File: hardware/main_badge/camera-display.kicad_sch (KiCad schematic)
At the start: 6 parts, among them J3 ILI9341 Display Module, J4 OV2640 Camera Module, Q1 2N7002

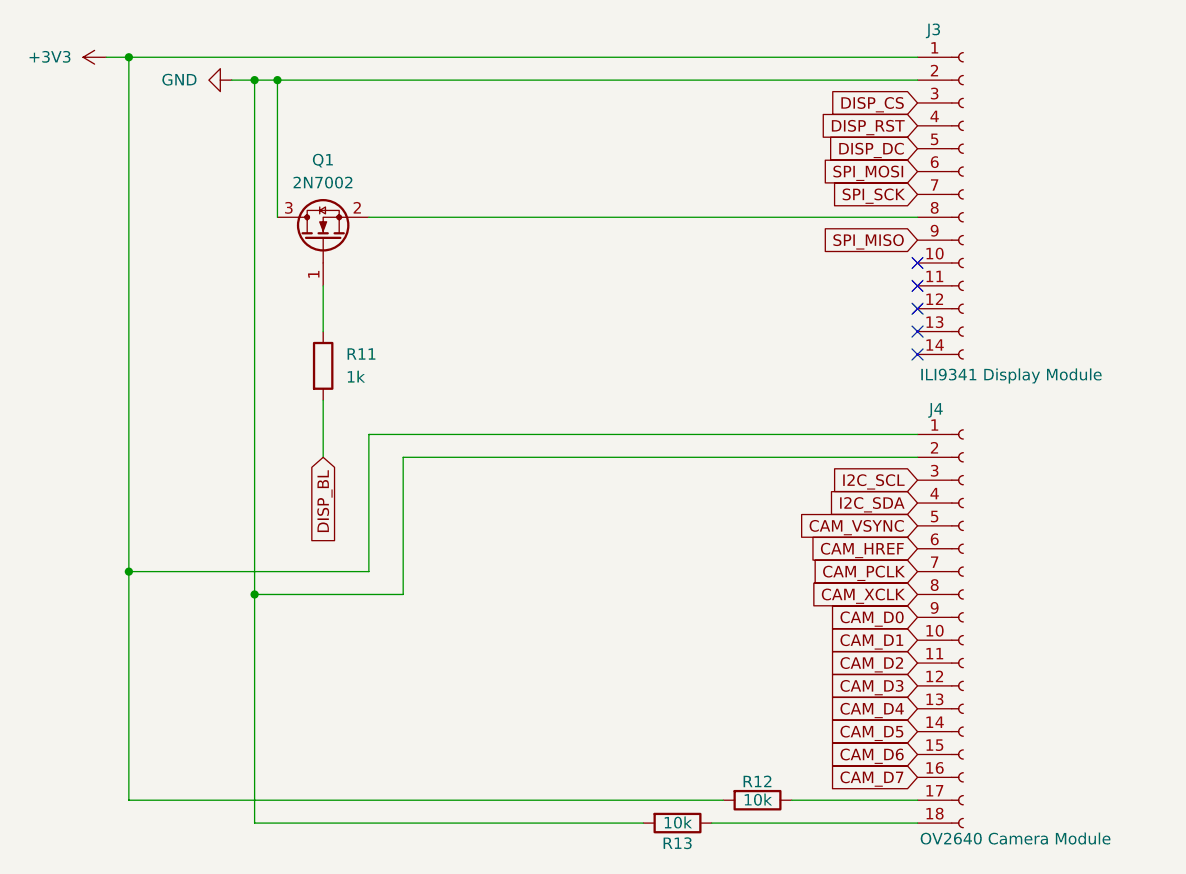
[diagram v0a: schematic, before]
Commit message: main board done except for placing LEDs and drawing ears... I think
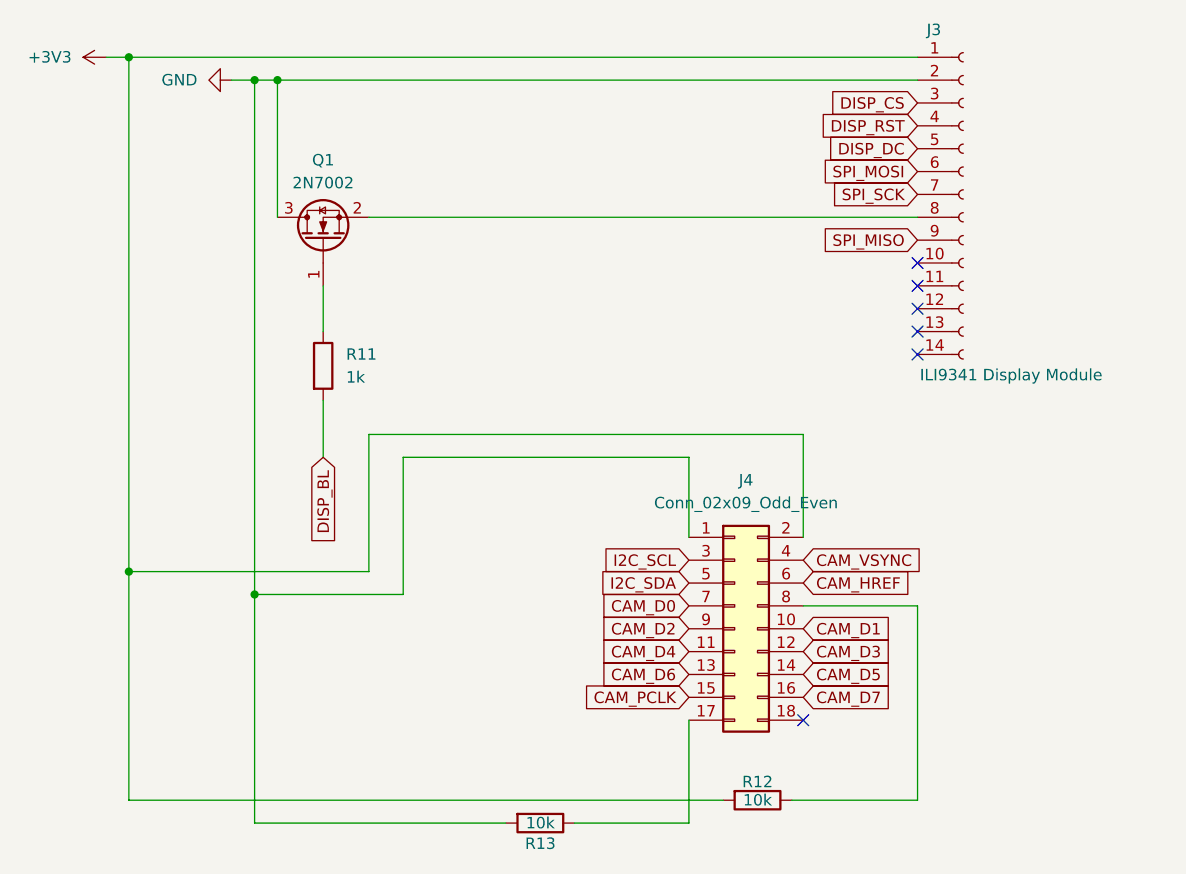
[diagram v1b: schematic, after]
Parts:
- removed J4: OV2640 Camera Module, Connector_PinSocket_2.54mm:PinSocket_1x18_P2.54mm_Vertical, symbol Connector:Conn_01x18_Socket
- added J4: Conn_02x09_Odd_Even, Connector_PinSocket_2.54mm:PinSocket_2x09_P2.54mm_Vertical, symbol Connector_Generic:Conn_02x09_Odd_Even
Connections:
- net +3V3: now also J4.2 (Pin_2)
- net CAM_D0: now also J4.7 (Pin_7)
- net CAM_D1: now also J4.10 (Pin_10)
- net CAM_D2: now also J4.9 (Pin_9)
- net CAM_D3: now also J4.12 (Pin_12)
- net CAM_D4: now also J4.11 (Pin_11)
- net CAM_D5: now also J4.14 (Pin_14)
- net CAM_D6: now also J4.13 (Pin_13)
- net CAM_D7: now also J4.16 (Pin_16)
- net CAM_HREF: now also J4.6 (Pin_6)
- net CAM_PCLK: now also J4.15 (Pin_15)
- net CAM_VSYNC: now also J4.4 (Pin_4)
- net GND: now also J4.1 (Pin_1)
- net I2C_SCL: now also J4.3 (Pin_3)
- net I2C_SDA: now also J4.5 (Pin_5)
- net at R12.1: now also J4.8 (Pin_8)
- net at R13.1: now also J4.17 (Pin_17)
- no-connect marks 5 -> 6
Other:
- moved on the sheet: R13
